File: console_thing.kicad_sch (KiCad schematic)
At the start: 74 parts, among them J1 Conn_01x03, SW1 SW_Push_45deg, SW2 SW_Push_45deg, SW3 SW_Push_45deg, SW4 SW_Push_45deg, SW5 SW_Push_45deg, SW6 SW_Push_45deg, SW7 SW_SPDT, U2 CH32V003FxPx

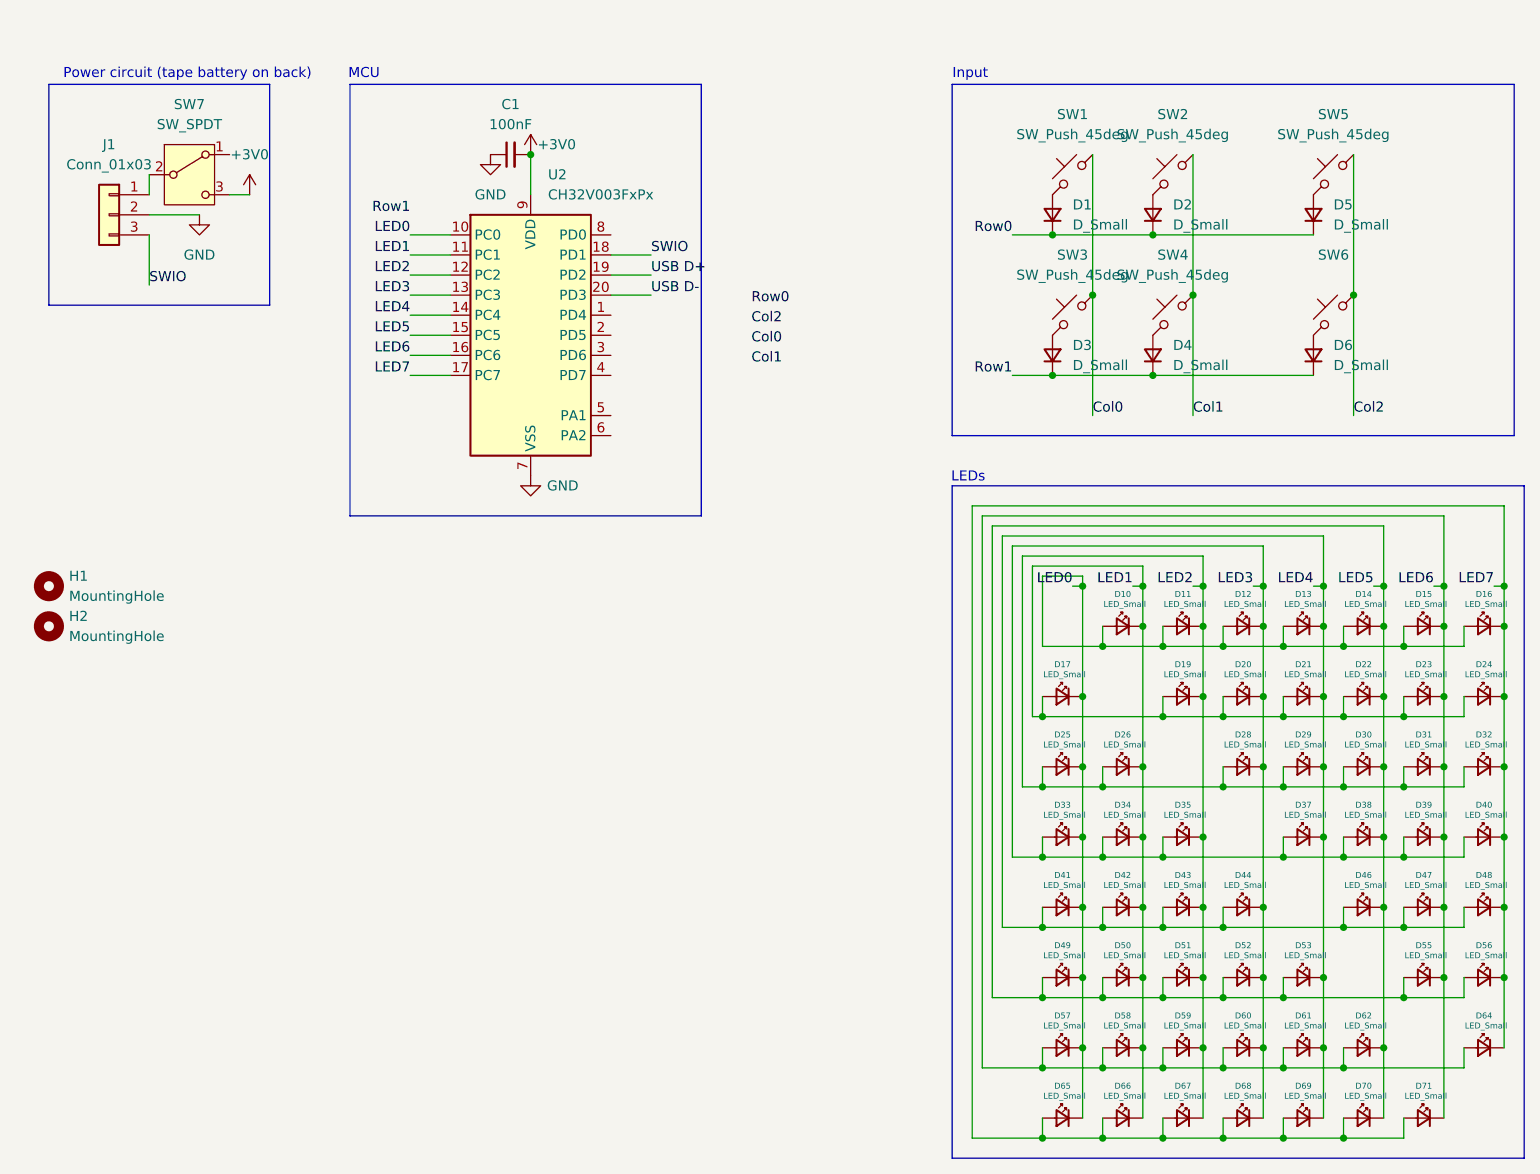
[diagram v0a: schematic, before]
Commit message: rerouted
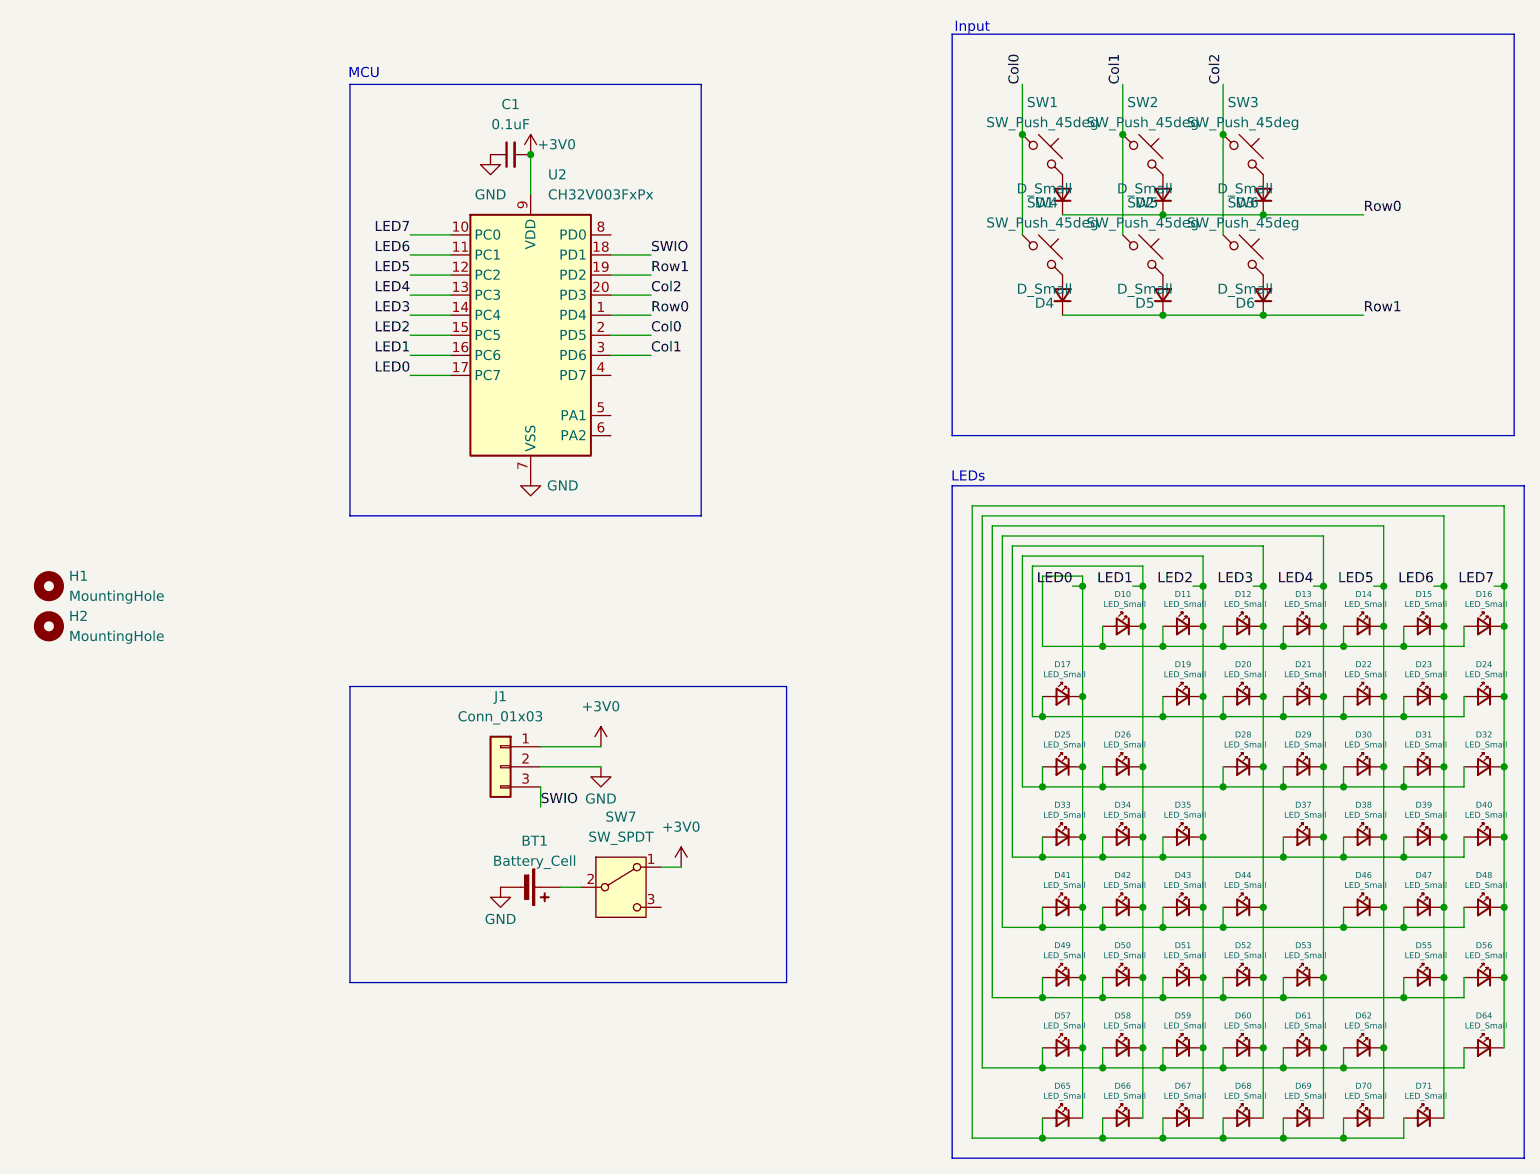
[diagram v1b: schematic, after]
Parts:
- added BT1: Battery_Cell, Battery:BatteryHolder_Keystone_1058_1x2032, symbol Device:Battery_Cell
- C1: value 100nF -> 0.1uF
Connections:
- net USB D+ is gone; now on net Row1: U2.19 (PD2)
- net USB D- is gone; now on net Col2: U2.20 (PD3)
- net +3V0: now also J1.1 (Pin_1), SW7.1 (A); no longer SW7.3 (C)
- net Col0: now also SW4.1, U2.2 (PD5); no longer SW3.1
- net Col1: now also SW5.1, U2.3 (PD6); no longer SW4.1
- net Col2: now also SW3.1; no longer SW5.1
- net GND: now also BT1.2 (-)
- net LED0: now also U2.17 (PC7); no longer U2.10 (PC0)
- net LED1: now also U2.16 (PC6); no longer U2.11 (PC1)
- net LED2: now also U2.15 (PC5); no longer U2.12 (PC2)
- net LED3: now also U2.14 (PC4); no longer U2.13 (PC3)
- net LED4: now also U2.13 (PC3); no longer U2.14 (PC4)
- net LED5: now also U2.12 (PC2); no longer U2.15 (PC5)
- net LED6: now also U2.11 (PC1); no longer U2.16 (PC6)
- net LED7: now also U2.10 (PC0); no longer U2.17 (PC7)
- net Row0: now also D3.1 (K), U2.1 (PD4); no longer D5.1 (K)
- net Row1: now also D5.1 (K); no longer D3.1 (K)
- net at SW7.2 (B): now also BT1.1 (+); no longer J1.1 (Pin_1)
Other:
- note removed: "Power circuit (tape battery on back)"
- moved on the sheet: D1, J1, SW1, SW7
